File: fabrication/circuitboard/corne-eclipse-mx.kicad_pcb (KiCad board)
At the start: 2 copper layers, 275.5 x 105.6 mm, 182 parts, among them J2 OLED, J4 OLED, SW1 SW_MX_HS, SW10 SW_MX_HS, SW11 SW_MX_HS, SW12 SW_MX_HS, SW13 SW_MX_HS, SW14 SW_MX_HS, SW15 SW_MX_HS, SW16 SW_MX_HS, SW17 SW_MX_HS, SW18 SW_MX_HS, SW2 SW_MX_HS, SW20 SW_MX_HS, SW21 SW_MX_HS, SW22 SW_MX_HS, SW23 SW_MX_HS, SW24 SW_MX_HS, SW25 SW_MX_HS, SW26 SW_MX_HS, SW27 SW_MX_HS, SW28 SW_MX_HS, SW29 SW_MX_HS, SW3 SW_MX_HS, SW30 SW_MX_HS, SW31 SW_MX_HS, SW32 SW_MX_HS, SW33 SW_MX_HS, SW34 SW_MX_HS, SW35 SW_MX_HS, SW36 SW_MX_HS, SW37 SW_MX_HS, SW38 SW_MX_HS, SW39 SW_MX_HS, SW4 SW_MX_HS, SW40 SW_MX_HS, SW42 SW_MX_HS, SW43 SW_MX_HS, SW44 SW_MX_HS, SW5 SW_MX_HS, SW6 SW_MX_HS, SW7 SW_MX_HS, SW8 SW_MX_HS, SW9 SW_MX_HS, U1 nice!nano, U2 nice!nano

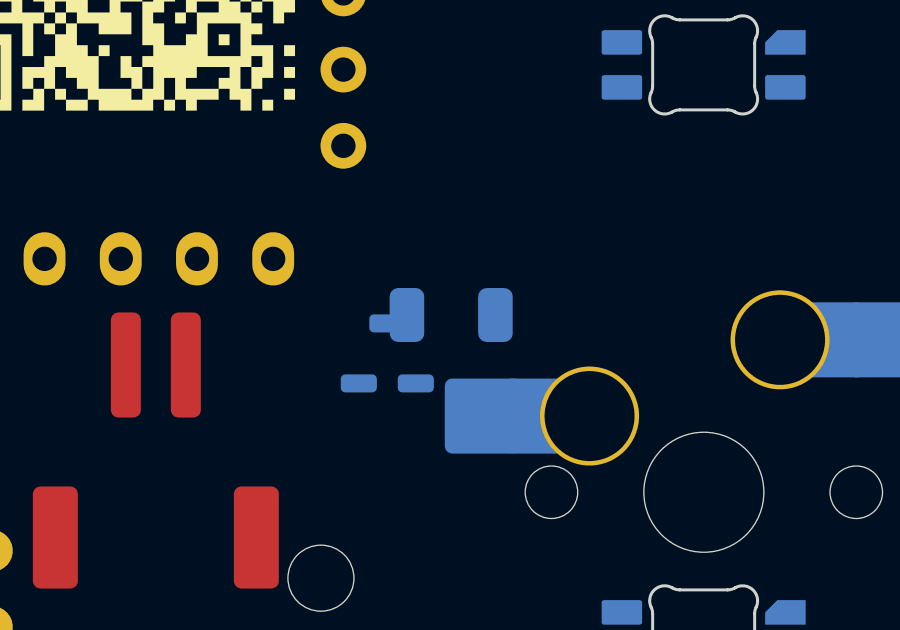
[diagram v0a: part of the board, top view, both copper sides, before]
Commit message: wip
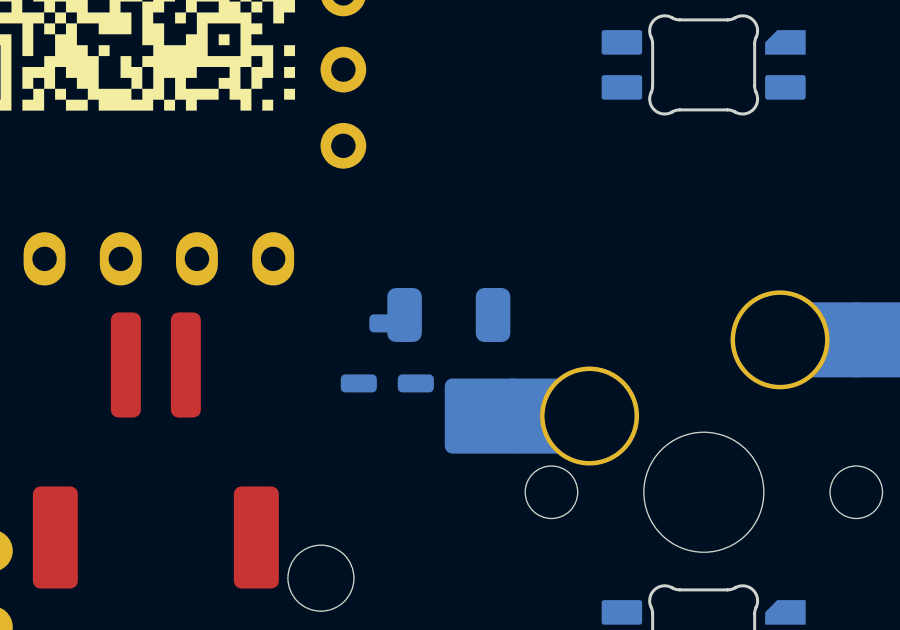
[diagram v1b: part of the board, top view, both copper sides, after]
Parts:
- moved R2 0.08 mm to (173.1, 64.5)
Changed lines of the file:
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@@
 	(footprint "Resistor_SMD:R_1206_3216Metric"
 		(layer "B.Cu")
-		(at 173.1925 64.5 180)
+		(at 173.1125 64.5 180)
 		(descr "10k Pull-up Resistor for MOSFET Gate")
 		(tags "resistor 1206")
